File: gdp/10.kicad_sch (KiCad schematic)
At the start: 8 parts, among them IC46 2732, IC47 HM6116, IC50 SCB2675

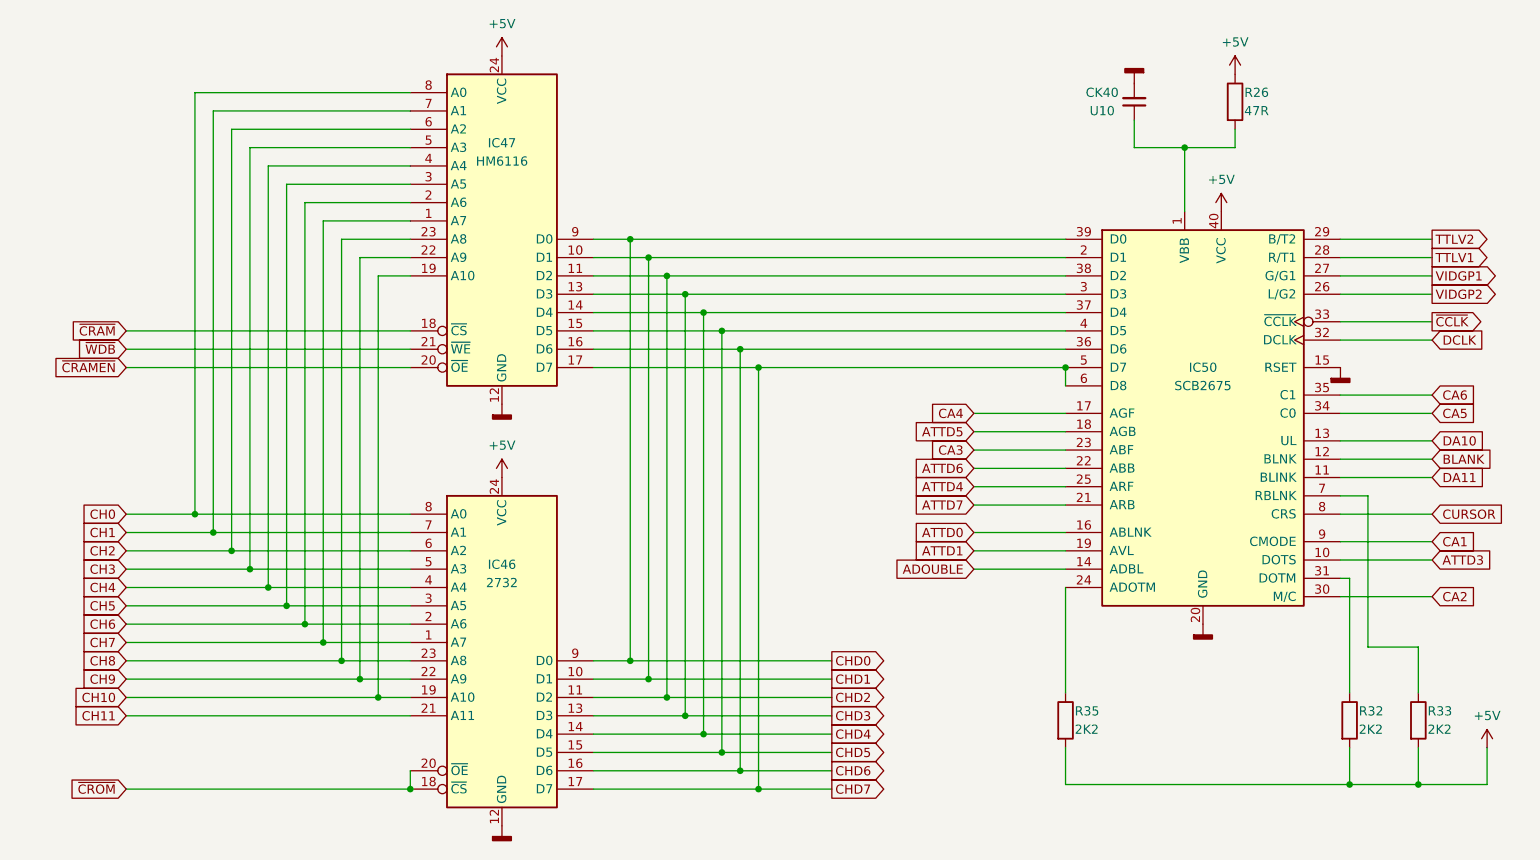
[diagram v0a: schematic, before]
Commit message: Fixes GND issue (R32)
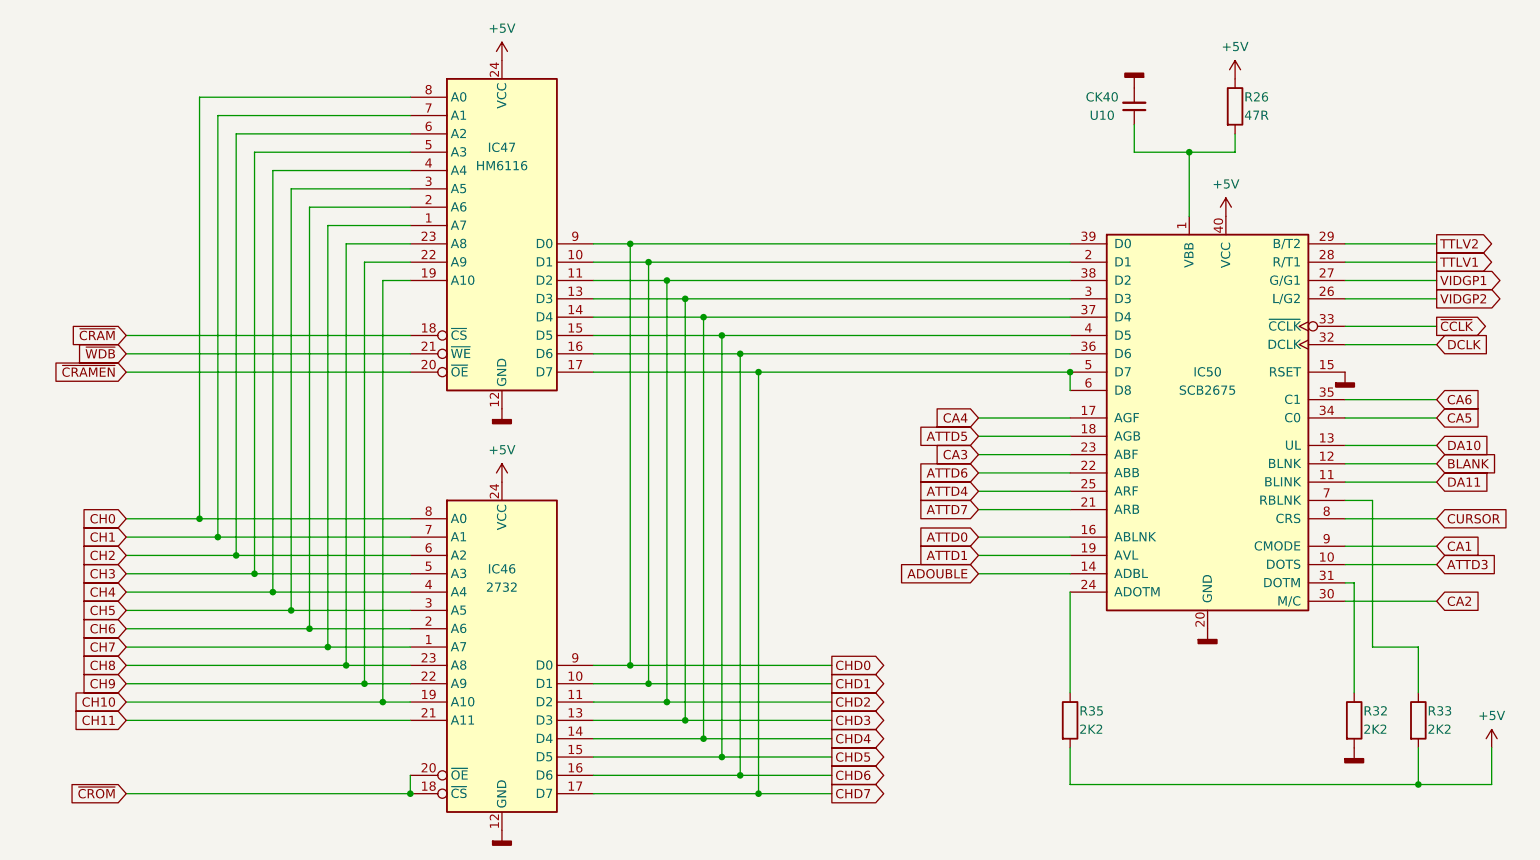
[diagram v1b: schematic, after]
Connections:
- net +5V: no longer R32.2
- net GNDD: now also R32.2
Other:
- moved on the sheet: CK40, IC46, IC47, IC50, R26, R32, R35
